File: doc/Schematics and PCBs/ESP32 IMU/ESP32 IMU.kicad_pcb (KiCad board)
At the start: 2 copper layers, 74 x 67.5 mm, 3 parts

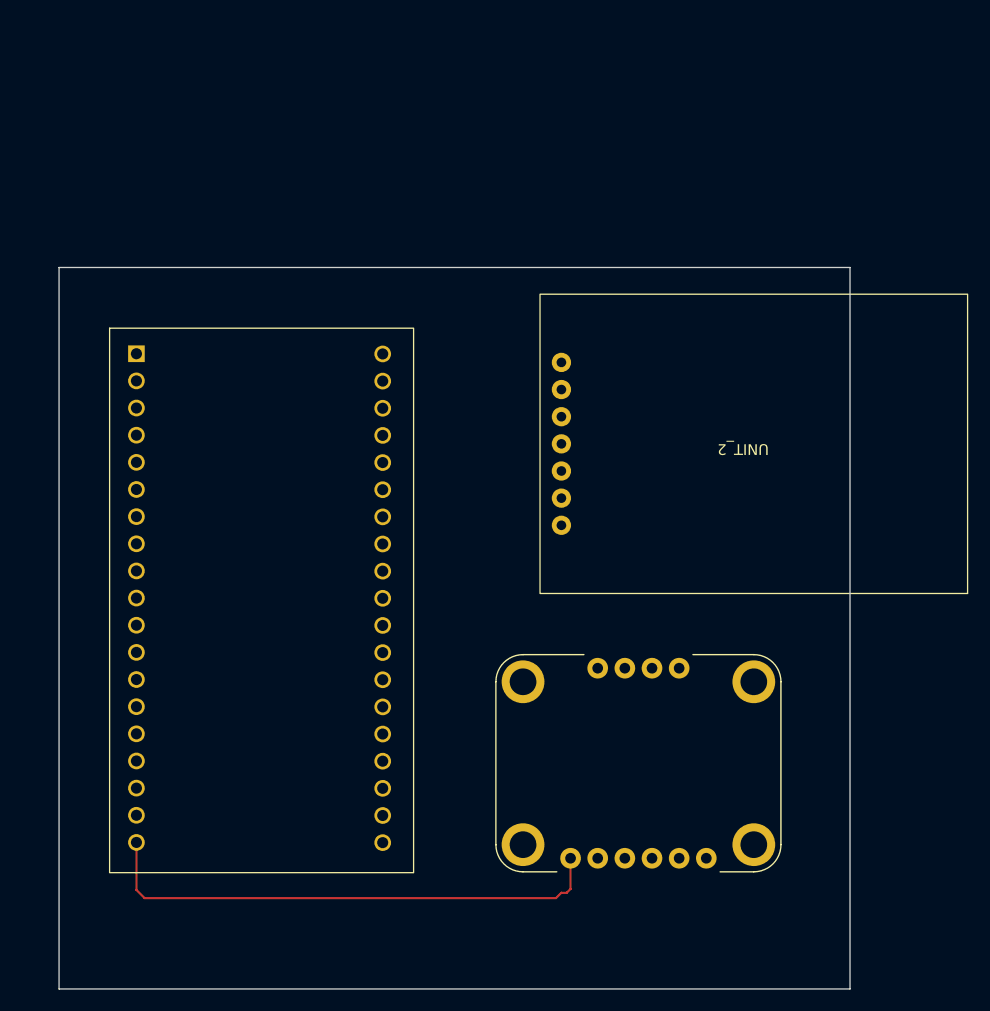
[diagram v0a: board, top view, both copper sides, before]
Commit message: Updated IMU PCB/Uploaded custom symbology
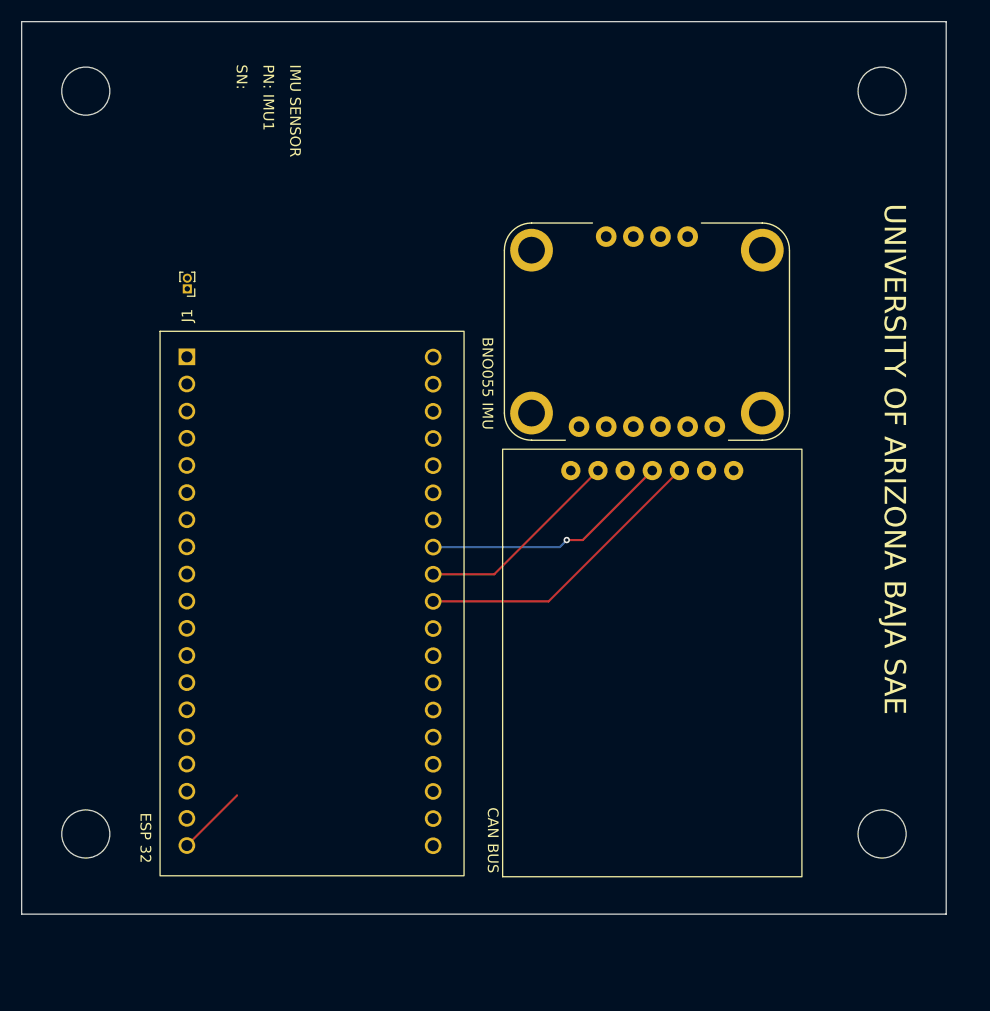
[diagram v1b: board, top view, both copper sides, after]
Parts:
- added J1: +5V, Connector_PinHeader_1.00mm:PinHeader_1x02_P1.00mm_Vertical, F.Cu at (117.5, 61.0)
- added REF**: MountingHole_4.5mm, MountingHole:MountingHole_4.5mm, F.Cu at (108.0, 42.5)
- added REF**: MountingHole_4.5mm, MountingHole:MountingHole_4.5mm, F.Cu at (182.5, 112.0)
- added REF**: MountingHole_4.5mm, MountingHole:MountingHole_4.5mm, F.Cu at (182.5, 42.5)
- added REF**: MountingHole_4.5mm, MountingHole:MountingHole_4.5mm, F.Cu at (108.0, 112.0)
- moved UNIT_3 40.4 mm to (160.5, 65.0)
- moved UNIT_2 21.3 mm to (161.0, 95.0), turned to 90 degrees
- moved UNIT_1 4.73 mm to (129.2, 86.3)
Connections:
- UNIT_2 pad 6: unconnected-(UNIT_2-GND-Pad6) -> GND
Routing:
- net +5V: track 48.6 -> 6.63 mm
- net Net-(UNIT_1-IO5): track 0.00 -> 28.1 mm
- net Net-(UNIT_1-IO19): track 0.00 -> 23.5 mm, vias 0 -> 1
- net Net-(UNIT_1-IO18): track 0.00 -> 19.4 mm
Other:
- board size 74 x 67.5 mm -> 86.5 x 83.5 mm
- board text added: "BNO055 IMU"
- board text added: "CAN BUS"
- board text added: "ESP 32"
- board text added: "GND"
- board text added: "IMU SENSOR"
- board text added: "PN: IMU1"
- board text added: "SN:"
- board text added: "UNIVERSITY OF ARIZONA BAJA SAE"

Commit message: Updated IMU PCB
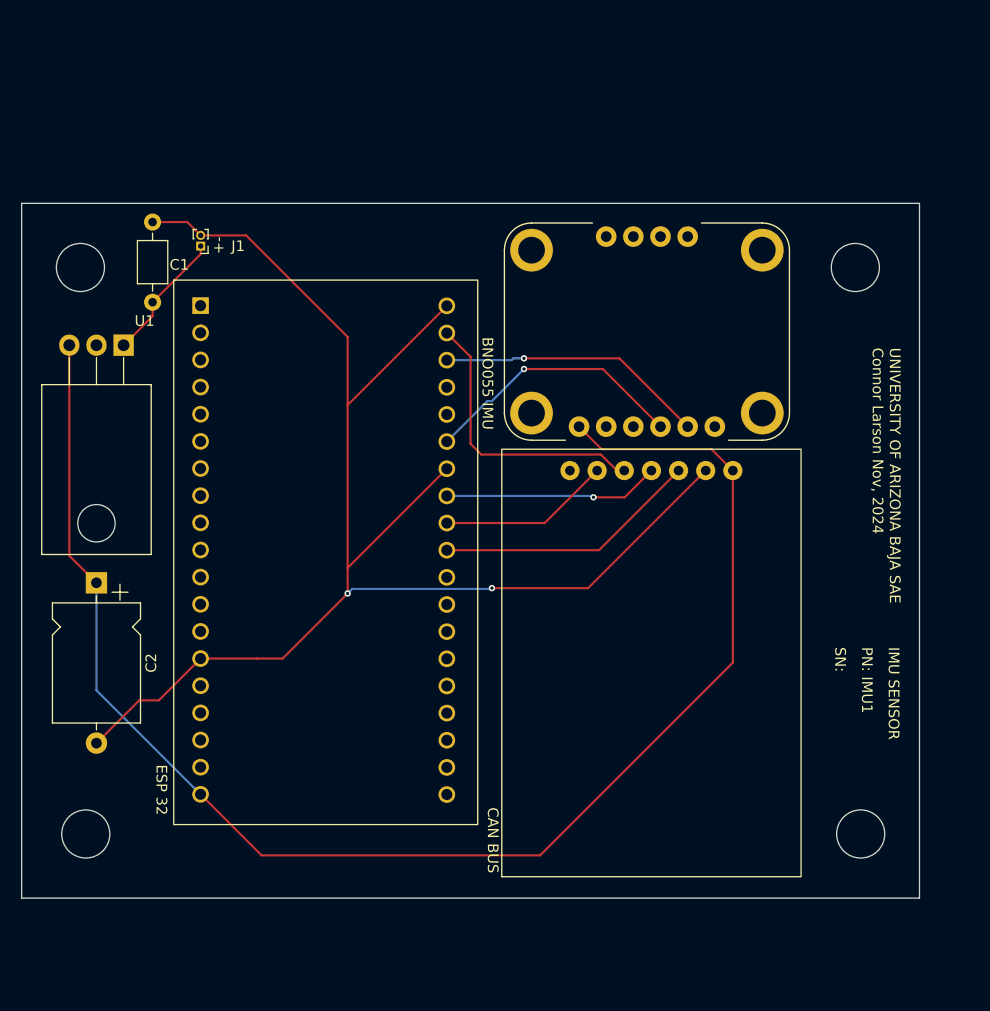
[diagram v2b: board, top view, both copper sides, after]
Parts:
- added C1: .33u, Capacitor_THT:C_Axial_L3.8mm_D2.6mm_P7.50mm_Horizontal, F.Cu at (114.2, 62.2)
- added C2: 22u, Capacitor_THT:CP_Axial_L11.0mm_D8.0mm_P15.00mm_Horizontal, F.Cu at (109.0, 88.5)
- added U1: BA50JC5T, Package_TO_SOT_THT:TO-220-3_Horizontal_TabDown, F.Cu at (111.5, 66.3)
- moved REF** 16.7 mm to (180.0, 59.0)
- moved REF** 16.5 mm to (107.5, 59.0)
- moved UNIT_1 4.96 mm to (130.5, 81.5)
- moved J1 4.19 mm to (118.8, 57.0)
- moved REF** 2.00 mm to (180.5, 112.0)
- moved UNIT_2 0.08 mm to (160.9, 95.0)
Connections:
- J1 pad 1: +5V -> Net-(J1-Pin_1)
- UNIT_1 pad J2-19: +5V -> +5v
- UNIT_2 pad 7: +5V -> +5v
- UNIT_3 pad 1: +5V -> +5v
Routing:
- net GND: track 0.00 -> 141.3 mm, vias 0 -> 2
- net +5v: track 0.00 -> 140.8 mm
- net Net-(UNIT_1-IO23): track 0.00 -> 26.7 mm
- net Net-(UNIT_1-IO22): track 0.00 -> 25.2 mm, vias 0 -> 1
- net Net-(UNIT_1-IO21): track 0.00 -> 25.0 mm, vias 0 -> 1
- net Net-(J1-Pin_1): track 0.00 -> 12.3 mm
- net +5V: track 6.63 -> 0.00 mm
- net Net-(UNIT_1-IO18): track 19.4 -> 16.1 mm
- net Net-(UNIT_1-IO5): track 28.1 -> 24.8 mm
- net Net-(UNIT_1-IO19): track 23.5 -> 20.2 mm
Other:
- board size 86.5 x 83.5 mm -> 84 x 65 mm
- board text added: "+-"
- board text added: "UNIVERSITY OF ARIZONA BAJA SAE Connor Larson Nov, 2024"
- board text removed: "GND"
- board text removed: "UNIVERSITY OF ARIZONA BAJA SAE"
